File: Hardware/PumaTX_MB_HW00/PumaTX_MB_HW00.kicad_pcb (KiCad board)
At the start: 4 copper layers, 130 x 40 mm, 106 parts, among them J100 FH12A-26S-0.5SH_55_, J101 FH12-12S-0.5SH_55_, J102 500334-0160, J103 500334-0160, J104 692122030100, J105 53398-0667, J300 U.FL-R-SMT-1_40_, J410 U.FL-R-SMT-1_40_, M130 Motor_DC, M140 Fan, Q130 ZXMN3B01F, Q140 ZXMN3B01F, Q200 UMH3NTN, Q201 UMH3NTN, U200 CP2105-F01-GMR, U300 ESP32-PICO-D4, U400 ESP32-PICO-D4, U402 E28-2G4M27S, U410 SX1280, U500 BQ24075RGTR, U510 MIC5528-3.3YMT-T5, U520 MIC5528-3.3YMT-T5, U530 MIC5528-3.3YMT-T5, Y410 NX2016SA-52MHZ-EXS00A-CS06016

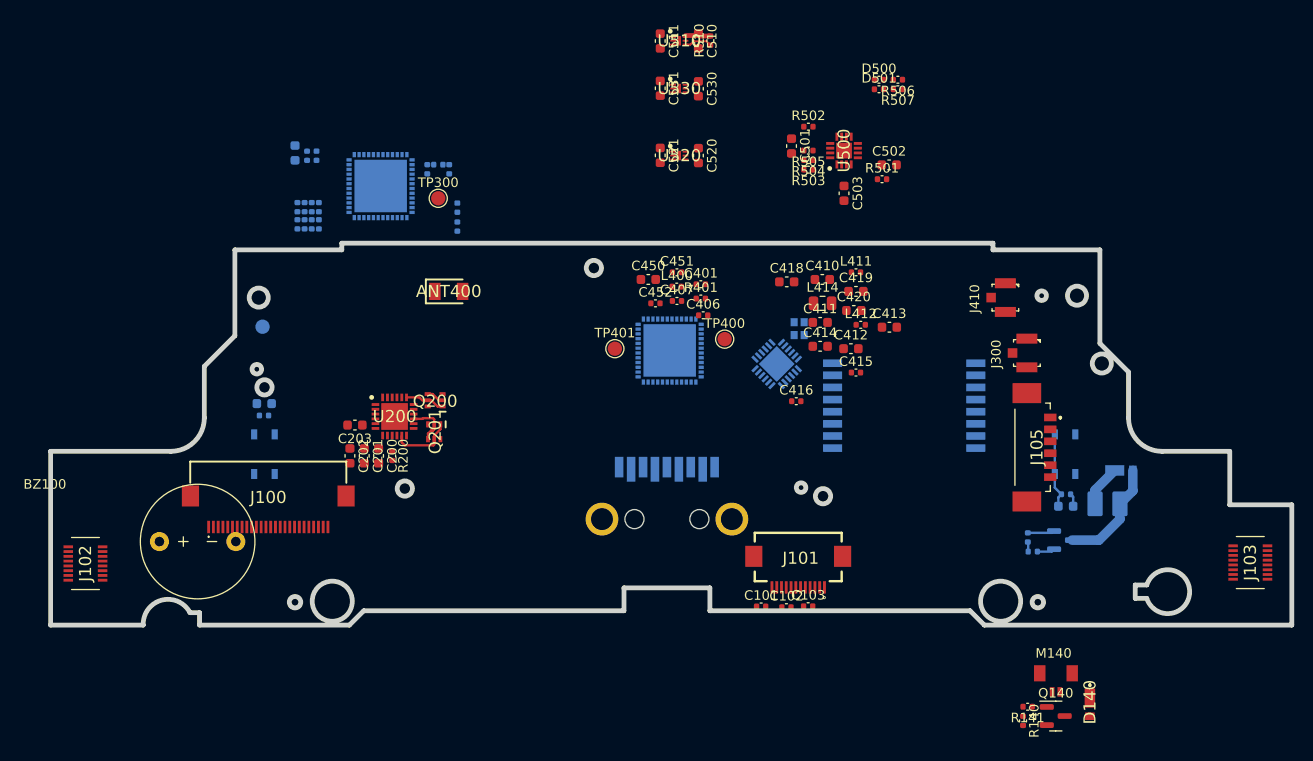
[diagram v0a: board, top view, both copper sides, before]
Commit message: Continued routing
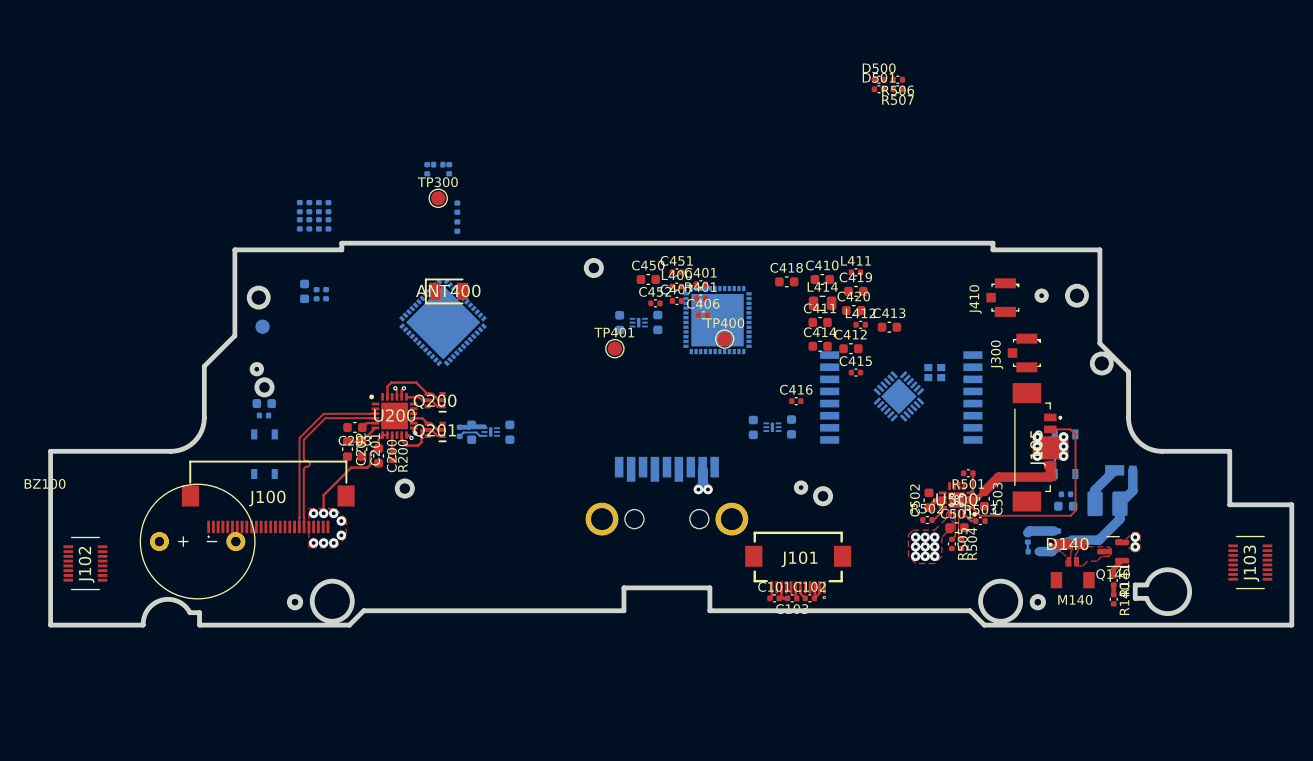
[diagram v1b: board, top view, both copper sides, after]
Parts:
- C510, C511, C520, C521, C530, C531, R510, U510, U520, U530: moved to B.Cu
- moved R510 48.7 mm to (124.2, 103.0)
- moved C510 47.4 mm to (125.5, 103.0)
- moved U510 45.5 mm to (127.5, 103.0), turned to 180 degrees
- moved C511 43.9 mm to (129.5, 103.0)
- moved R505 43.9 mm to (175.8, 114.7), turned to -90 degrees
- moved C501 43.6 mm to (176.3, 113.0), turned to 0 degrees
- moved R504 43.3 mm to (176.8, 114.7), turned to -90 degrees
- moved R502 43.0 mm to (173.2, 112.2)
- moved R503 41.0 mm to (178.8, 112.3), turned to 0 degrees
- moved U500 38.5 mm to (176.3, 110.1), turned to 180 degrees
- moved C531 38.0 mm to (159.0, 102.5)
- moved U530 36.8 mm to (157.0, 102.5), turned to 180 degrees
- moved C530 35.9 mm to (155.0, 102.5)
- moved C502 35.4 mm to (173.4, 110.1), turned to 90 degrees
- moved C503 35.2 mm to (179.2, 110.0)
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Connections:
- D130 pad 1: /HAPTIC_HS -> /VSYS
- D140 pad 1: /FAN_HS -> /VSYS
- M130 pad 1: /HAPTIC_HS -> /VSYS
- M140 pad 1: /FAN_HS -> /VSYS
- R506 pad 1: /SYS -> /VSYS
- R507 pad 1: /SYS -> /VSYS
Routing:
- net VBUS: track 0.00 -> 114.2 mm, vias 0 -> 19
- net /BATTERY_TEMP: track 0.00 -> 22.5 mm
- net GND: track 3.25 -> 24.2 mm, vias 0 -> 14
- net /D+: track 0.00 -> 18.3 mm
- net /D-: track 0.00 -> 18.3 mm
- net /VBAT: track 0.00 -> 10.6 mm
- net /VSYS: track 2.79 -> 8.96 mm
- net /PUMATX_DTR: track 1.82 -> 7.79 mm
- net /HAPTIC_HS: track 4.35 -> 0.00 mm
- net /C2: track 7.95 -> 4.15 mm
- net /3V45: track 0.00 -> 3.53 mm
- net /SYSOFF: track 0.00 -> 2.88 mm
- net /TMR: track 0.00 -> 2.85 mm
- net /BQ_CE: track 0.00 -> 2.15 mm
- net /ILIM: track 0.00 -> 2.03 mm
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- added copper zone on F.Cu, net /FAN_LS
- added copper zone on F.Cu, net /VSYS
- added copper zone on F.Cu, net GND
- added copper zone on In1.Cu, net GND
- added copper zone on F.Cu, net VBUS

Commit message: quick esp32 update
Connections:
- U300 pad 49: (no net) -> GND
- U400 pad 49: (no net) -> GND
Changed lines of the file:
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@@
     (property "Sheetname" "")
     (attr smd)
-    (fp_text reference "U300" (at -0.341 0.132 135) (layer "B.SilkS")
-      (effects (font (size 1.27 1.27) (thickness 0.254)) (justify mirror))
-    )
-    (fp_text value "ESP32-PICO-D4" (at -0.341 0.132 135) (layer "B.SilkS") hide
-      (effects (font (size 1.27 1.27) (thickness 0.254)) (justify mirror))
-    )
-    (fp_text user "${REFERENCE}" (at -0.341 0.132 135) (layer "B.Fab")
+    (fp_text reference "U300" (at -0.341 0.132 315) (layer "B.SilkS")
+      (effects (font (size 1.27 1.27) (thickness 0.254)) (justify mirror))
+    )
+    (fp_text value "ESP32-PICO-D4" (at -0.341 0.132 315) (layer "B.SilkS") hide
+      (effects (font (size 1.27 1.27) (thickness 0.254)) (justify mirror))
+    )
+    (fp_text user "${REFERENCE}" (at -0.341 0.132 315) (layer "B.Fab")
       (effects (font (size 1.27 1.27) (thickness 0.254)) (justify mirror))
     )
     (fp_circle (center -3.991 2.825) (end -3.991 2.78788) (layer "B.SilkS") (width 0.2) (fill none))
-    (fp_line (start -3.5 -3.5) (end -3.5 3.5) (layer "B.Fab") (width 0.2))
     (fp_line (start -3.5 3.5) (end 3.5 3.5) (layer "B.Fab") (width 0.2))
     (fp_line (start 3.5 3.5) (end 3.5 -3.5) (layer "B.Fab") (width 0.2))
     (fp_line (start 3.5 -3.5) (end -3.5 -3.5) (layer "B.Fab") (width 0.2))
+    (fp_line (start -3.5 -3.5) (end -3.5 3.5) (layer "B.Fab") (width 0.2))
     (pad "1" smd rect (at -3.3 2.75 45) (size 0.35 0.55) (layers "B.Cu" "B.Paste" "B.Mask")
       (net 2 "+3V3") (pinfunction "VDDA") (pintype "power_in"))
@@
     (pad "48" smd rect (at -2.75 3.3 135) (size 0.35 0.55) (layers "B.Cu" "B.Paste" "B.Mask")
       (net 81 "unconnected-(U300-Pad48)") (pinfunction "CAP1") (pintype "bidirectional+no_connect"))
-    (pad "49" smd rect (at -0.006 0.013 45) (size 5.5 5.5) (layers "B.Cu" "B.Paste" "B.Mask"))
+    (pad "49" smd rect (at -0.006 0.013 45) (size 5.5 5.5) (layers "B.Cu" "B.Paste" "B.Mask")
+      (net 1 "GND") (pinfunction "GND") (pintype "power_in"))
     (model "C:/Users/Nico/Desktop/Component_lib/Hardware/SamacSys_Parts.3dshapes/ESP32-PICO-V3.stp"
       (offset (xyz 0 0 0))
@@
     (property "Sheetname" "")
     (attr smd)
-    (fp_text reference "U400" (at -0.341 0.132) (layer "B.SilkS")
-      (effects (font (size 1.27 1.27) (thickness 0.254)) (justify mirror))
-    )
-    (fp_text value "ESP32-PICO-D4" (at -0.341 0.132) (layer "B.SilkS") hide
-      (effects (font (size 1.27 1.27) (thickness 0.254)) (justify mirror))
-    )
-    (fp_text user "${REFERENCE}" (at -0.341 0.132) (layer "B.Fab")
+    (fp_text reference "U400" (at -0.341 0.132 180) (layer "B.SilkS")
+      (effects (font (size 1.27 1.27) (thickness 0.254)) (justify mirror))
+    )
+    (fp_text value "ESP32-PICO-D4" (at -0.341 0.132 180) (layer "B.SilkS") hide
+      (effects (font (size 1.27 1.27) (thickness 0.254)) (justify mirror))
+    )
+    (fp_text user "${REFERENCE}" (at -0.341 0.132 180) (layer "B.Fab")
       (effects (font (size 1.27 1.27) (thickness 0.254)) (justify mirror))
     )
     (fp_circle (center -3.991 2.825) (end -3.991 2.78788) (layer "B.SilkS") (width 0.2) (fill none))
+    (fp_line (start 3.5 3.5) (end 3.5 -3.5) (layer "B.Fab") (width 0.2))
     (fp_line (start -3.5 -3.5) (end -3.5 3.5) (layer "B.Fab") (width 0.2))
+    (fp_line (start 3.5 -3.5) (end -3.5 -3.5) (layer "B.Fab") (width 0.2))
     (fp_line (start -3.5 3.5) (end 3.5 3.5) (layer "B.Fab") (width 0.2))
-    (fp_line (start 3.5 -3.5) (end -3.5 -3.5) (layer "B.Fab") (width 0.2))
-    (fp_line (start 3.5 3.5) (end 3.5 -3.5) (layer "B.Fab") (width 0.2))
     (pad "1" smd rect (at -3.3 2.75 270) (size 0.35 0.55) (layers "B.Cu" "B.Paste" "B.Mask")
       (net 39 "-3V3") (pinfunction "VDDA") (pintype "power_in"))
@@
     (pad "48" smd rect (at -2.75 3.3) (size 0.35 0.55) (layers "B.Cu" "B.Paste" "B.Mask")
       (net 115 "unconnected-(U400-Pad48)") (pinfunction "CAP1") (pintype "bidirectional+no_connect"))
-    (pad "49" smd rect (at -0.006 0.013 270) (size 5.5 5.5) (layers "B.Cu" "B.Paste" "B.Mask"))
+    (pad "49" smd rect (at -0.006 0.013 270) (size 5.5 5.5) (layers "B.Cu" "B.Paste" "B.Mask")
+      (net 1 "GND") (pinfunction "GND") (pintype "power_in"))
     (model "C:/Users/Nico/Desktop/Component_lib/Hardware/SamacSys_Parts.3dshapes/ESP32-PICO-V3.stp"
       (offset (xyz 0 0 0))

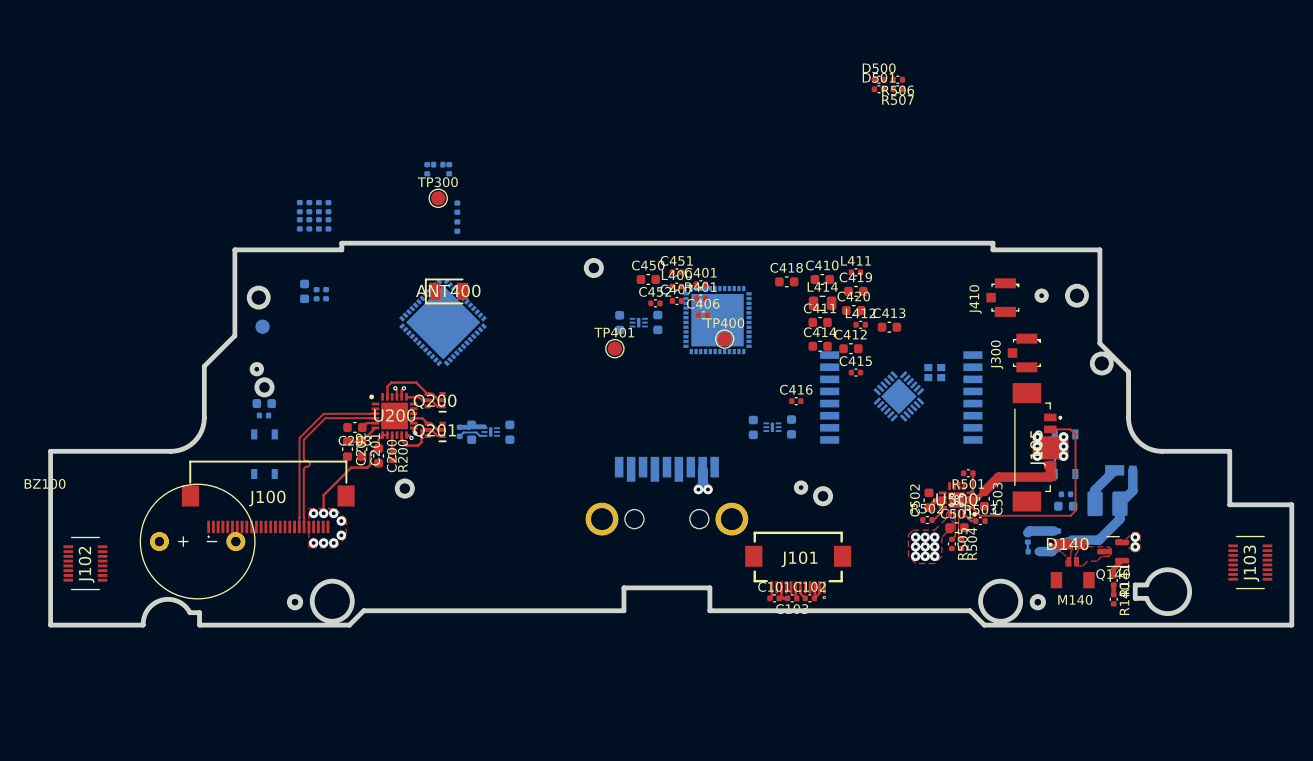
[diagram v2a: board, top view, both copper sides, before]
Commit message: working on routing / placement
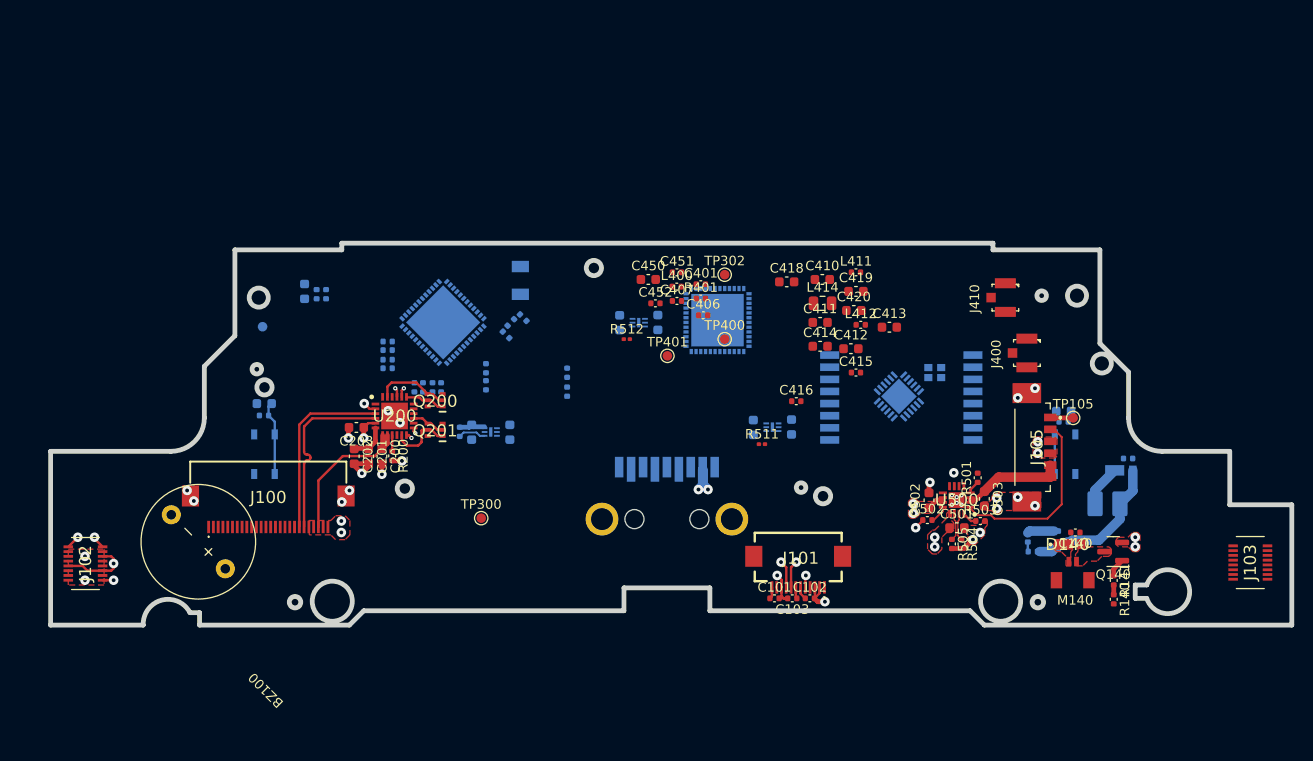
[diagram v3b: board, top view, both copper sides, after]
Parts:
- removed ANT400: 2450AT18A100E, Component_lib:ANTC3216X140N
- removed D500, D501: LED, Capacitor_SMD:C_0402_1005Metric
- removed J300: U.FL-R-SMT-1_40_, Component_lib:u.fl
- removed R506, R507: 1k5, Capacitor_SMD:C_0402_1005Metric
- added ANT300: 2450AT18A100E, Component_lib:ANTC3216X140N, B.Cu at (130.6, 87.1)
- added C130: 100n, Capacitor_SMD:C_0402_1005Metric, B.Cu at (194.2, 105.8)
- added C140: 100n, Capacitor_SMD:C_0402_1005Metric, F.Cu at (188.7, 113.5)
- added J400: U.FL-R-SMT-1_40_, Component_lib:u.fl, F.Cu at (183.7, 94.7)
- added R305: 120k, Capacitor_SMD:C_0402_1005Metric, B.Cu at (127.0, 96.3)
- added R306: 470k, Capacitor_SMD:C_0402_1005Metric, B.Cu at (127.0, 98.1)
- added R511: 0, Capacitor_SMD:C_0201_0603Metric, F.Cu at (155.9, 104.2)
- added R512: 0, Capacitor_SMD:C_0201_0603Metric, F.Cu at (141.8, 93.2)
- added TP105: BAT_WHITE, TestPoint:TestPoint_Pad_D1.0mm, F.Cu at (188.5, 101.5)
- added TP302: CRSF, TestPoint:TestPoint_Pad_D1.0mm, F.Cu at (152.0, 86.5)
- TP300, TP301, TP401: footprint TestPoint:TestPoint_Pad_D1.5mm -> TestPoint:TestPoint_Pad_D1.0mm
- TP400: value TestPoint -> ELRS_CHIP_PU; footprint TestPoint:TestPoint_Pad_D1.5mm -> TestPoint:TestPoint_Pad_D1.0mm
- moved TP300 33.8 mm to (126.5, 112.0)
- moved R302 23.4 mm to (122.3, 98.3), turned to 90 degrees
- moved R301 22.4 mm to (119.5, 98.3), turned to 90 degrees
- moved C301 21.4 mm to (120.4, 98.3)
- moved C302 21.4 mm to (121.4, 98.3)
- moved C300 20.8 mm to (135.5, 98.8)
- moved R300 20.8 mm to (135.5, 96.8)
- moved C306 19.2 mm to (129.1, 92.8), turned to -45 degrees
- moved L300 18.2 mm to (129.6, 91.5), turned to -135 degrees
- moved R304 18.0 mm to (116.7, 96.3), turned to 0 degrees
- moved C307 17.4 mm to (130.9, 91.0), turned to -45 degrees
- moved R303 15.8 mm to (116.7, 93.5), turned to 0 degrees
- moved C304 15.5 mm to (116.7, 95.4), turned to 180 degrees
- moved C303 15.0 mm to (116.7, 94.4), turned to 180 degrees
- moved C120 9.95 mm to (187.5, 100.8)
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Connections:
- J100 pad 10: /LED_ANODE -> /LED
- J100 pad 14: /LED_CATHODE -> GND
- U410 pad 25: (no net) -> GND
- U520 pad 4: /LED -> /AUX_EN
- U530 pad 4: /LED -> /AUX_EN
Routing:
- net VBUS: track 114.2 -> 103.5 mm, vias 19 -> 6
- net +3V3: track 2.76 -> 12.1 mm, vias 0 -> 3
- net /C1: track 0.00 -> 7.77 mm
- net /BATTERY_TEMP: track 22.5 -> 19.4 mm
- net /DISPLAY_SCL: track 0.00 -> 2.98 mm, vias 0 -> 1
- net /DISPLAY_SDA: track 0.00 -> 2.88 mm, vias 0 -> 1
- net /BATTERY_WHITE: track 0.00 -> 2.42 mm
- net /PUMATX_SDA: track 0.00 -> 1.41 mm, vias 0 -> 1
- net /PUMATX_SCL: track 0.00 -> 1.35 mm, vias 0 -> 1
- net /LEFT_POT: track 0.00 -> 1.15 mm, vias 0 -> 1
- net GND: track 24.2 -> 25.3 mm, vias 14 -> 36
- net /D-: track 18.3 -> 19.1 mm
- net /D+: track 18.3 -> 19.2 mm
- net /BQ_CE: track 2.15 -> 1.41 mm
- net /VSYS: vias 0 -> 2

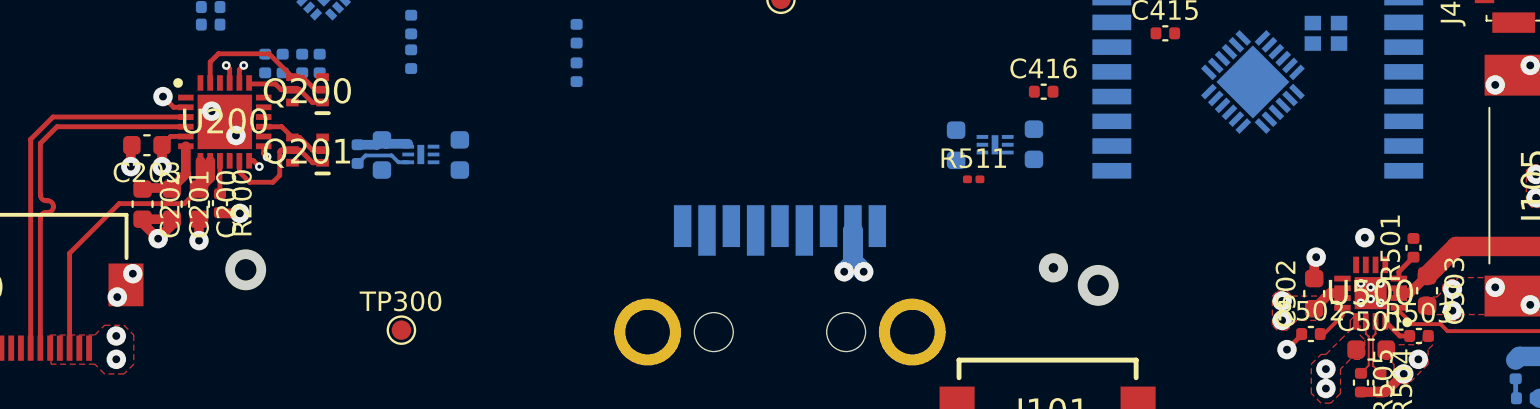
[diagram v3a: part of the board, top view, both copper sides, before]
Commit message: Quick update
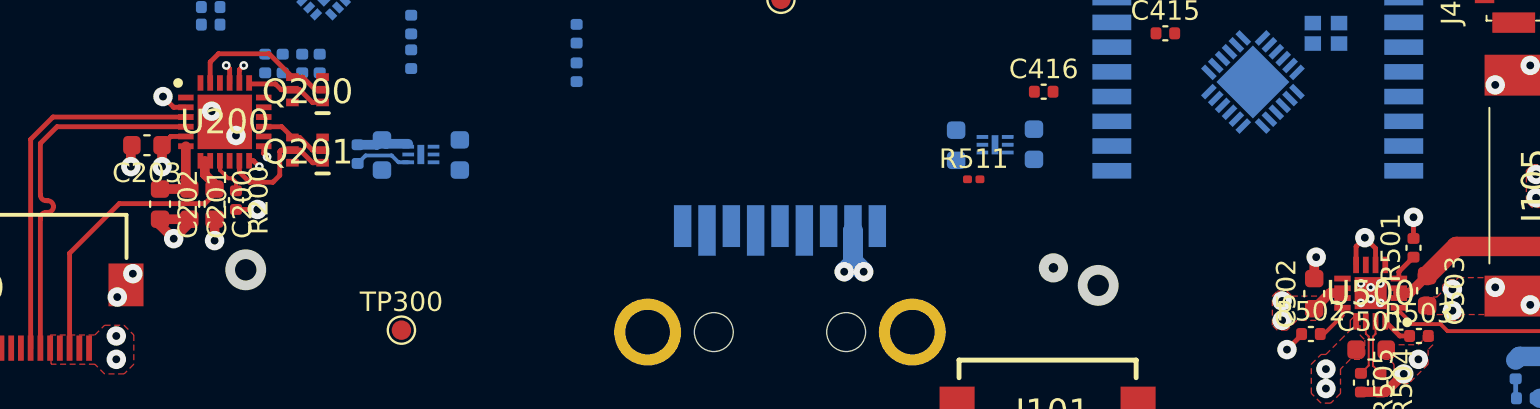
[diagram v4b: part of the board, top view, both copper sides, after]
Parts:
- moved C201 0.90 mm to (115.6, 105.5)
- moved C202 0.90 mm to (114.1, 105.5)
- moved R200 0.84 mm to (118.0, 105.3)
- moved C200 0.80 mm to (116.9, 105.5)
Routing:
- net GND: track 25.3 -> 29.7 mm, vias 36 -> 37
- net VBUS: track 103.5 -> 103.0 mm
